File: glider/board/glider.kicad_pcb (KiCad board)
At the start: 2 copper layers, 131 x 33 mm, 9 parts, among them J1 Conn_01x05_Socket, J4 Conn_01x02, J5 Conn_01x02, U1 TPS613221ADBV 5V converter, U2 ESP32-DevKitC

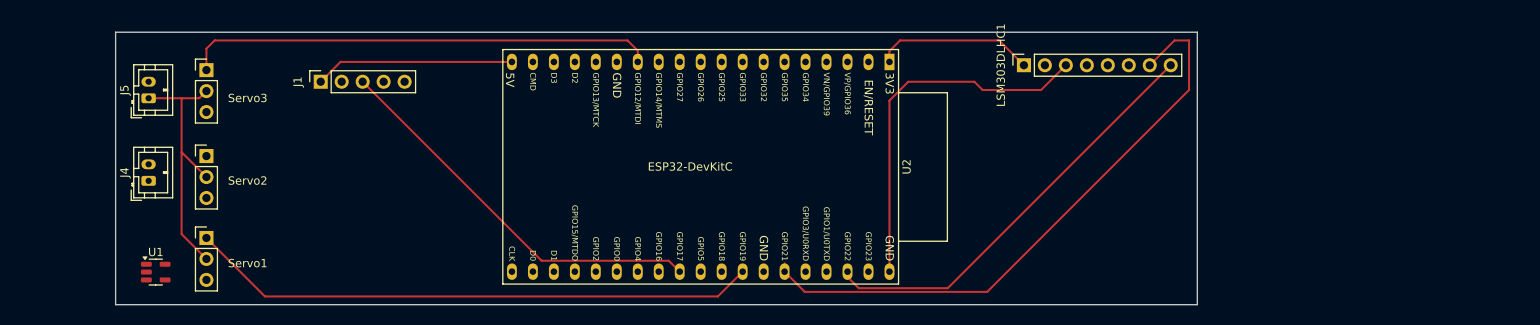
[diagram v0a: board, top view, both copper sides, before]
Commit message: Update board
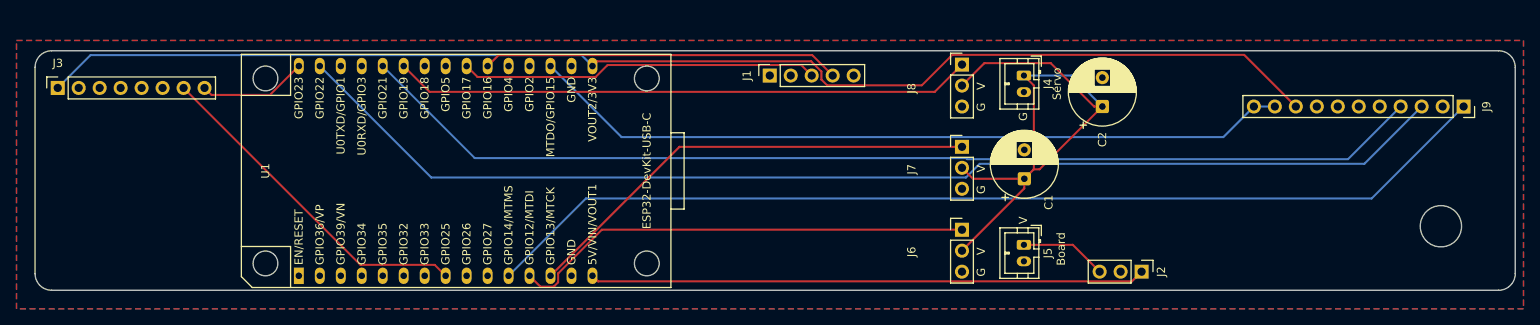
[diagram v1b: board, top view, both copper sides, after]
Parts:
- removed LSM303DLHC1: Conn_01x08_Socket, Connector_PinSocket_2.54mm:PinSocket_1x08_P2.54mm_Vertical
- removed Servo1, Servo2, Servo3: Conn_01x03_Pin, Connector_PinHeader_2.54mm:PinHeader_1x03_P2.54mm_Vertical
- removed U2: ESP32-DevKitC, PCM_Espressif:ESP32-DevKitC
- added C1: C_Polarized, Capacitor_THT:CP_Radial_D8.0mm_P3.50mm, F.Cu at (202.1, 71.8)
- added C2: C_Polarized, Capacitor_THT:CP_Radial_D8.0mm_P3.50mm, F.Cu at (211.5, 63.0)
- added J2: 5V buck boost, Connector_PinHeader_2.54mm:PinHeader_1x03_P2.54mm_Vertical, F.Cu at (216.2, 83.0)
- added J3: LSM303DLHC1, Connector_PinSocket_2.54mm:PinSocket_1x08_P2.54mm_Vertical, F.Cu at (85.0, 60.8)
- added J6: Servo 1, Connector_PinHeader_2.54mm:PinHeader_1x03_P2.54mm_Vertical, F.Cu at (194.5, 77.9)
- added J7: Servo 2, Connector_PinHeader_2.54mm:PinHeader_1x03_P2.54mm_Vertical, F.Cu at (194.5, 67.9)
- added J8: Servo 3, Connector_PinHeader_2.54mm:PinHeader_1x03_P2.54mm_Vertical, F.Cu at (194.5, 57.9)
- added J9: Si4713_FM_transmitter, Connector_PinSocket_2.54mm:PinSocket_1x11_P2.54mm_Vertical, F.Cu at (255.2, 63.0)
- J1: value Conn_01x05_Socket -> GT-U7 GPS
- J4, J5: value Conn_01x02 -> Li-Ion Molex
- U1: value TPS613221ADBV 5V converter -> ESP32-DevKit-USB-C; footprint Package_TO_SOT_SMD:SOT-23-5 -> boards:ESP32-DevKit-USB-C
- moved J5 107.5 mm to (202.0, 79.8), turned to -90 degrees
- moved J4 106.8 mm to (202.0, 59.2), turned to -90 degrees
- moved J1 54.4 mm to (171.2, 59.2)
- moved U1 17.3 mm to (114.2, 83.5), turned to 90 degrees
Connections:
- J1 pad 1: 5V -> /5v
- J1 pad 3: D17 -> /GPIO17
- J1 pad 4: D16 -> /GPIO16
- J4 pad 1: +3V3 -> 3v7servo
- J5 pad 1: +4V -> 3v7board
- U1 pad 1: +3V3 -> unconnected-(U1-CHIP_PU-Pad1)
- U1 pad 2: GND -> unconnected-(U1-SENSOR_VP/GPIO36/ADC1_CH0-Pad2)
- U1 pad 4: 5V -> unconnected-(U1-VDET_1/GPIO34/ADC1_CH6-Pad4)
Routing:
- net /3v3: track 0.00 -> 158.3 mm
- net /GPIO22: track 0.00 -> 142.6 mm
- net /GPIO21: track 0.00 -> 130.6 mm
- net /GPIO14: track 0.00 -> 124.2 mm
- net /GPIO15: track 0.00 -> 92.8 mm
- net 3v7servo: track 0.00 -> 76.2 mm
- net D21: track 73.1 -> 0.00 mm
- net /GPIO19: track 0.00 -> 70.3 mm
- net D19: track 69.1 -> 0.00 mm
- net /5v: track 0.00 -> 67.3 mm
- net D12: track 57.1 -> 0.00 mm
- net /GPIO12: track 0.00 -> 56.4 mm
- net /GPIO13: track 0.00 -> 56.3 mm
- net D22: track 52.2 -> 0.00 mm
- net D17: track 47.9 -> 0.00 mm
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- added copper zone on B.Cu, net GND
- added copper zone on F.Cu, net GND
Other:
- board size 131 x 33 mm -> 179.2 x 29 mm
- board text added: "3v3"
- board text added: "3v7"
- board text added: "5v"
- board text added: "Board"
- board text added: "G"
- board text added: "GND"
- board text added: "GT-U7 GPS"
- board text added: "LSM303DLHC1 accelerometer"
- board text added: "Servo"
- board text added: "Servo 1 GPIO 12"
- board text added: "Servo 2 GPIO 13"
- board text added: "Servo 3 GPIO 19"
- board text added: "Si4713 FM transmitter"
- board text added: "V"
